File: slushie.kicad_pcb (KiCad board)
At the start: 2 copper layers, 99.1 x 99.1 mm, 103 parts, among them SW1 SPST, SW2 SPST, SW3 SPST, U1 LM2575, U2 LPC1769 LPCXpresso

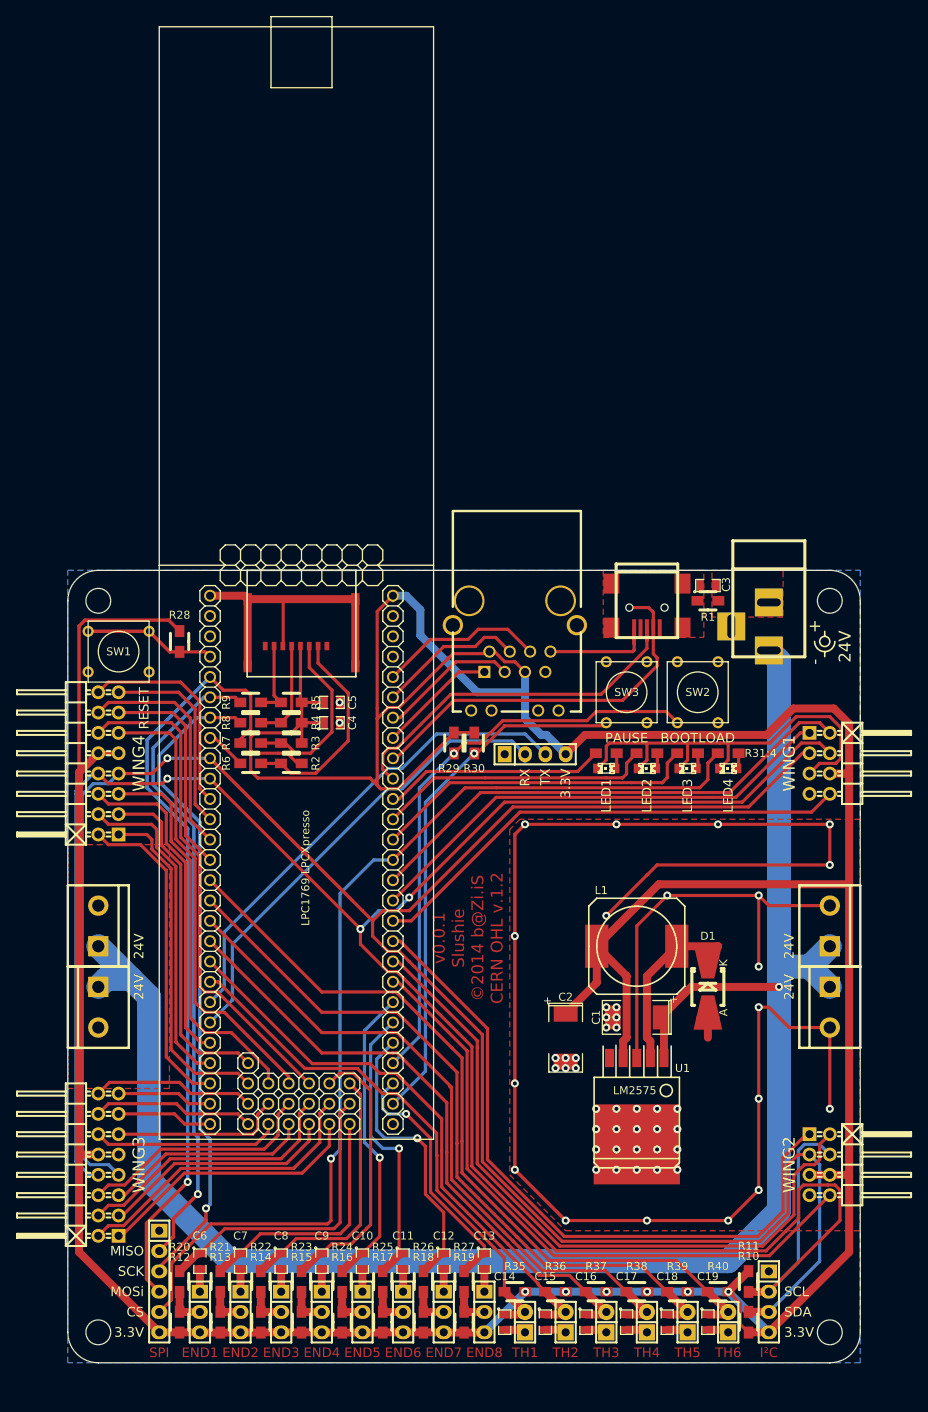
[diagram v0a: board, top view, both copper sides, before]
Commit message: clean
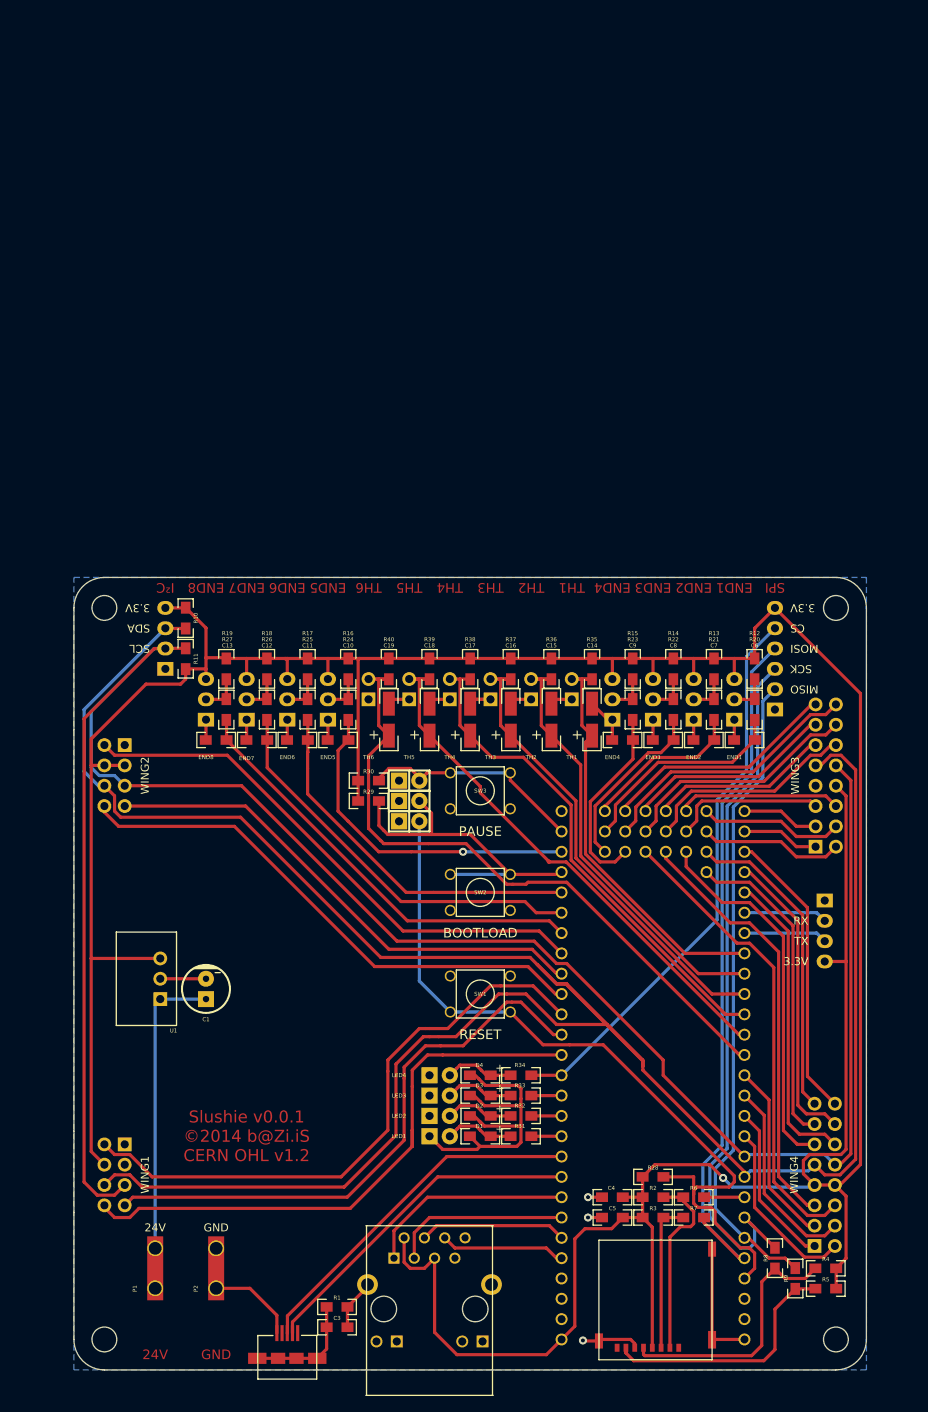
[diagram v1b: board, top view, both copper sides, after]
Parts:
- removed C2: CP, SMD_Packages:SMD-2512_Pol
- removed D5: LED, LEDs:LED-0805
- removed L1: 330µH, Inductors:SELF-WE-PD-XXL
- removed the Nylon Only at (132.7, 149.2)
- removed the Nylon Only at (132.7, 57.8)
- removed the Nylon Only at (224.2, 57.8)
- removed the Nylon Only at (224.2, 149.2)
- removed POWER1: BARREL_JACK, Connect:BARREL_JACK
- removed WINGPWR1, WINGPWR2, WINGPWR3, WINGPWR4: WINGPWR, Connect:bornier2
- added BOOT1: CONN_2, Pin_Headers:Pin_Header_Straight_1x02, F.Cu at (171.6, 82.8)
- added LED1: CONN_2, Pin_Headers:Pin_Header_Straight_1x02, F.Cu at (175.4, 124.7)
- added LED2: CONN_2, Pin_Headers:Pin_Header_Straight_1x02, F.Cu at (175.4, 122.2)
- added LED3: CONN_2, Pin_Headers:Pin_Header_Straight_1x02, F.Cu at (175.4, 119.6)
- added LED4: CONN_2, Pin_Headers:Pin_Header_Straight_1x02, F.Cu at (175.4, 117.1)
- added Nylon Only: 3-1mm, Local:MountingHole_3-1mm, F.Cu at (224.9, 58.7)
- added Nylon Only: 3-1mm, Local:MountingHole_3-1mm, F.Cu at (133.5, 58.7)
- added Nylon Only: 3-1mm, Local:MountingHole_3-1mm, F.Cu at (133.5, 150.1)
- added Nylon Only: 3-1mm, Local:MountingHole_3-1mm, F.Cu at (224.9, 150.1)
- added P1: CONN_1, Local:TabRA, F.Cu at (139.8, 141.2)
- added P2: CONN_1, Local:TabRA, F.Cu at (147.4, 141.2)
- added PAUSE1: CONN_2, Pin_Headers:Pin_Header_Straight_1x02, F.Cu at (171.6, 80.3)
- added RESET1: CONN_2, Pin_Headers:Pin_Header_Straight_1x02, F.Cu at (171.6, 85.3)
- C1: value CP -> 22µF; footprint SMD_Packages:SMD-2512_Pol -> Capacitors_ThroughHole:Capacitor5x11RM2.5
- C10, C11, C12, C13, C3, C4, C5, C6, C7, C8, C9: footprint SMD_Packages:SMD-0805 -> Local:0805C
- C14, C15, C16, C17, C18, C19: footprint SMD_Packages:SMD-0805 -> Local:EIA3216
- D1: value 1N5818 -> LED; footprint Diodes_SMD:Diode-Universal-SMB-SMC_Handsoldering -> Local:0805LED
- D2: footprint LEDs:LED-0805 -> 0805LED
- D3, D4: footprint LEDs:LED-0805 -> Local:0805LED
- END1, END2, END3, END4, END5, END6, END7, END8: footprint Pin_Headers:Pin_Header_Straight_1x03 -> Local:Pin_Header_Right_Angle_1x03
- ETHERNET1: footprint Connect:RJ45_TRANSFO -> Local:MJF12T3L-KF06B3YG-0808
- R1, R10, R11, R12, R13, R14, R15, R16, R17, R18, R19, R2, R20, R21, R22, R23, R24, R25, R26, R27, R28, R29, R3, R30, R31, R32, R33, R34, R35, R36, R37, R38, R39, R4, R40, R5, R6, R7, R8, R9: footprint Resistors_SMD:Resistor_SMD0805_HandSoldering -> Local:0805R
- SD1: footprint SD:MICRO_SD_HINGE_AMP -> MICRO_SD
- SW1, SW2, SW3: footprint Discret:SW_PUSH_SMALL -> Local:Tactswitch
- TH1, TH2, TH3, TH4, TH5, TH6: footprint Pin_Headers:Pin_Header_Straight_1x02 -> Local:Pin_Header_Angled_2x01
- U1: value LM2575 -> TR05S; footprint SMD_Packages:TO-263-5 -> Local:TR05S
- U2: footprint LPCXpresso_boards.mod:LPCXPRESSO_LPC1769 -> LPCXPRESSO_LPC1769
- USB1: footprint Connect:USB_MINI_B -> Local:USB_MICRO_B
- WING1, WING2: footprint Pin_Headers:Pin_Header_Angled_2x04 -> Socket_Strips:Socket_Strip_Angled_2x04
- WING3, WING4: footprint Pin_Headers:Pin_Header_Angled_2x08 -> Socket_Strips:Socket_Strip_Angled_2x08
- moved U2 140.6 mm to (213.5, 150.1), turned to 90 degrees
- moved R10 112.7 mm to (143.6, 59.9), turned to 90 degrees
- moved I2C1 112.1 mm to (141.1, 62.5), turned to 90 degrees
- moved SPI1 109.5 mm to (217.3, 65.0), turned to 90 degrees
- moved R12 108.8 mm to (214.8, 66.3), turned to 270 degrees
- moved SD1 108.0 mm to (202.1, 152.7), turned to 180 degrees
- moved USB1 106.1 mm to (156.3, 153.9), turned to 0 degrees
- moved R11 104.9 mm to (143.6, 65.0), turned to 270 degrees
- moved C3 103.7 mm to (162.6, 148.6)
- moved WING4 103.3 mm to (223.5, 129.5), turned to 270 degrees
- moved R13 102.4 mm to (209.7, 66.3), turned to 270 degrees
- moved WING1 102.0 mm to (134.7, 129.5), turned to 90 degrees
- moved WING3 102.0 mm to (223.6, 79.6), turned to 270 degrees
- moved END1 101.6 mm to (212.2, 70.1), turned to 90 degrees
- moved R20 101.4 mm to (214.8, 71.4), turned to 270 degrees
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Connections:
- net +24V renamed Net-(C1-Pad1)
- D1 pad 1: GND -> Net-(D1-Pad1)
- D1 pad 2: Net-(D1-Pad2) -> GND
- R31 pad 2: Net-(D2-Pad1) -> Net-(D1-Pad1)
- R32 pad 2: Net-(D3-Pad1) -> Net-(D2-Pad1)
- R33 pad 2: Net-(D4-Pad1) -> Net-(D3-Pad1)
- R34 pad 2: Net-(D5-Pad1) -> Net-(D4-Pad1)
- U1 pad 2: Net-(D1-Pad2) -> GND
- U1 pad 3: GND -> +3.3V
- U2 pad 42: /PWM1 -> /PWM2
- U2 pad 43: /PWM2 -> /PWM1
- U2 pad 48: /END4 -> /END7
- U2 pad 49: /END5 -> /END6
- U2 pad 50: /END6 -> /END5
- U2 pad 52: /END7 -> /END4
- WING1 pad 1: /PWM2 -> (no net)
- WING1 pad 2: /PWM1 -> /PWM0
- WING1 pad 3: /SDA -> GND
- WING1 pad 4: /SCL -> +3.3V
- WING1 pad 5: GND -> /SCL
- WING1 pad 6: +3.3V -> /SDA
- WING1 pad 7: (no net) -> /PWM1
- WING1 pad 8: /PWM0 -> /PWM2
- WING2 pad 1: /PWM5 -> (no net)
- WING2 pad 2: /PWM4 -> /PWM3
- WING2 pad 3: /SDA -> +3.3V
- WING2 pad 4: /SCL -> +3.3V
- WING2 pad 5: +3.3V -> /SCL
- WING2 pad 6: +3.3V -> /SDA
- WING2 pad 7: (no net) -> /PWM4
- WING2 pad 8: /PWM3 -> /PWM5
- WING3 pad 1: /EN3 -> /EN0
- WING3 pad 10: +3.3V -> /SCL
- WING3 pad 11: /DIR1 -> /STP2
- WING3 pad 12: /EN1 -> /EN2
- WING3 pad 13: /STP1 -> /DIR2
- WING3 pad 14: /DIR0 -> /STP3
- WING3 pad 15: /EN0 -> /EN3
- WING3 pad 16: /STP0 -> /DIR3
- WING3 pad 2: /DIR3 -> /STP0
- WING3 pad 3: /DIR2 -> /STP1
- WING3 pad 4: /STP3 -> /DIR0
- WING3 pad 5: /STP2 -> /DIR1
- WING3 pad 6: /EN2 -> /EN1
- WING3 pad 7: /SDA -> GND
- WING3 pad 8: /SCL -> +3.3V
- WING3 pad 9: GND -> /SDA
- WING4 pad 1: /EN7 -> /EN4
- WING4 pad 10: +3.3V -> /SCL
- WING4 pad 11: /DIR5 -> /STP6
- WING4 pad 12: /EN5 -> /EN6
- WING4 pad 13: /STP5 -> /DIR6
- WING4 pad 14: /DIR4 -> /STP7
- WING4 pad 15: /EN4 -> /EN7
- WING4 pad 16: /STP4 -> /DIR7
- WING4 pad 2: /DIR7 -> /STP4
- WING4 pad 3: /DIR6 -> /STP5
- WING4 pad 4: /STP7 -> /DIR4
- WING4 pad 5: /STP6 -> /DIR5
- WING4 pad 6: /EN6 -> /EN5
- WING4 pad 7: /SDA -> +3.3V
- WING4 pad 8: /SCL -> +3.3V
- WING4 pad 9: +3.3V -> /SDA
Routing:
- net GND: track 534.2 -> 130.6 mm, vias 53 -> 3
- net Net-(C1-Pad1): track 225.0 -> 42.5 mm, vias 1 -> 0
- net +3.3V: track 613.5 -> 468.6 mm, vias 6 -> 1
- net /RESET: track 16.6 -> 98.0 mm
- net /LED4: track 126.6 -> 70.7 mm, vias 1 -> 0
- net /TX: track 60.9 -> 10.5 mm
- net /RX: track 60.1 -> 10.5 mm
- net /PAUSE: track 66.1 -> 28.5 mm, vias 1 -> 0
- net /LED3: track 41.2 -> 3.78 mm
- net /SCL: track 298.9 -> 266.8 mm, vias 3 -> 0
- net /BOOT: track 72.5 -> 40.9 mm, vias 1 -> 0
- net /LED2: track 34.7 -> 3.78 mm
- net /TH4: track 95.4 -> 68.4 mm
- net /SDA: track 276.1 -> 302.3 mm, vias 1 -> 0
- net /TH3: track 88.5 -> 62.9 mm
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- removed copper zone on F.Cu, net GND
- removed copper zone on F.Cu, net Net-(C3-Pad1)
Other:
- outline, holes or cut-outs redrawn
- net class Default: trace_width 0.4318 -> 0.4
- board text added: "GND"
- board text added: "MOSI"
- board text added: "Slushie v0.0.1 ©2014 b@Zi.iS CERN OHL v1.2"
- board text removed: "+"
- board text removed: "-"
- board text removed: "LED1"
- board text removed: "LED2"
- board text removed: "LED3"
- board text removed: "LED4"
- board text removed: "LPC1769 LPCXpresso"
- board text removed: "MOSi"
- board text removed: "R31:4"
- board text removed: "v0.0.1 Slushie ©2014 b@Zi.iS CERN OHL v.1.2"
